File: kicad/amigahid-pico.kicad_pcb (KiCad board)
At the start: 2 copper layers, 80 x 76.2 mm, 60 parts, among them J1 Amiga keyboard connector, J2 Conn_02x05_Top_Bottom, J3 Conn_02x05_Top_Bottom, J4 Conn_01x06, J5 Conn_01x04, Q1 BSS138, Q10 BSS138, Q11 BSS138, Q12 BSS138, Q13 BSS138, Q14 BSS138, Q15 BSS138, Q16 BSS138, Q17 BSS138, Q2 BSS138, Q3 BSS138, Q4 BSS138, Q5 BSS138, Q6 BSS138, Q7 BSS138, Q8 BSS138, Q9 BSS138, U1 Pico

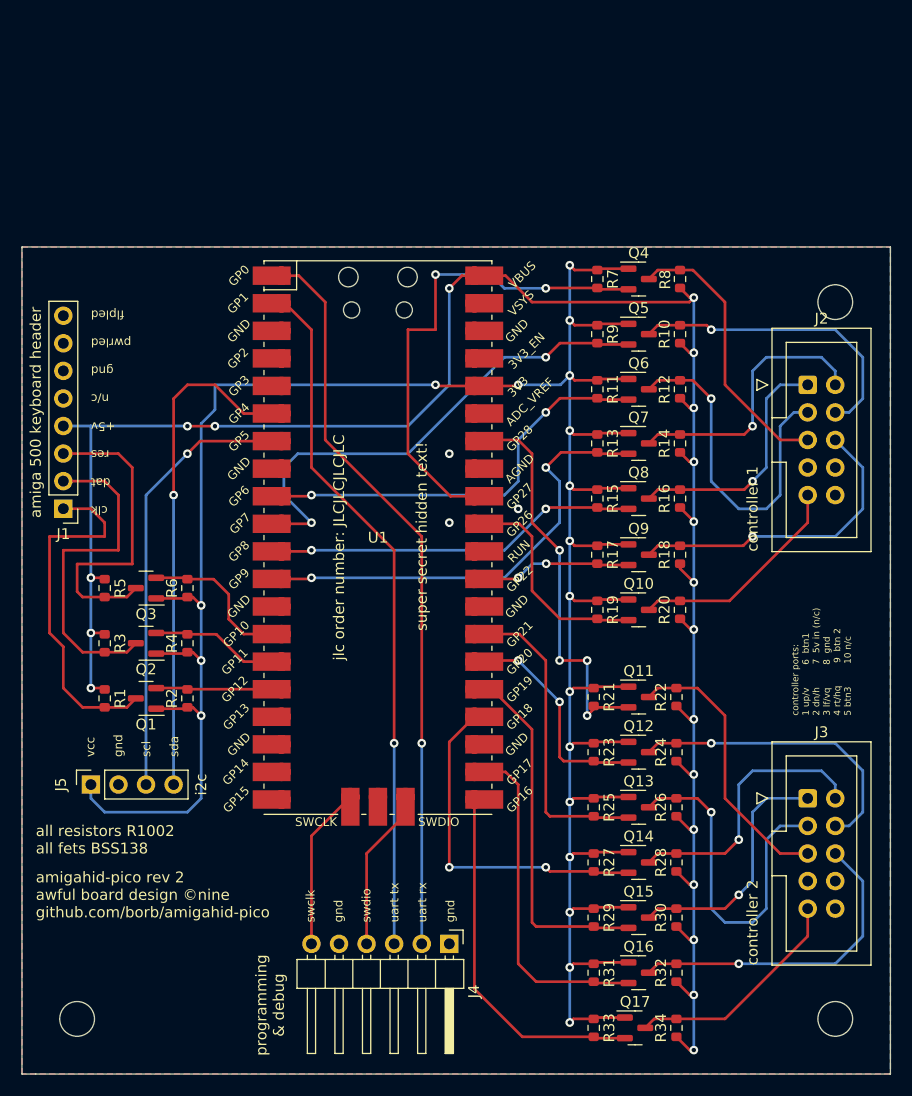
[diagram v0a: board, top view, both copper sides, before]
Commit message: pcb rev 4
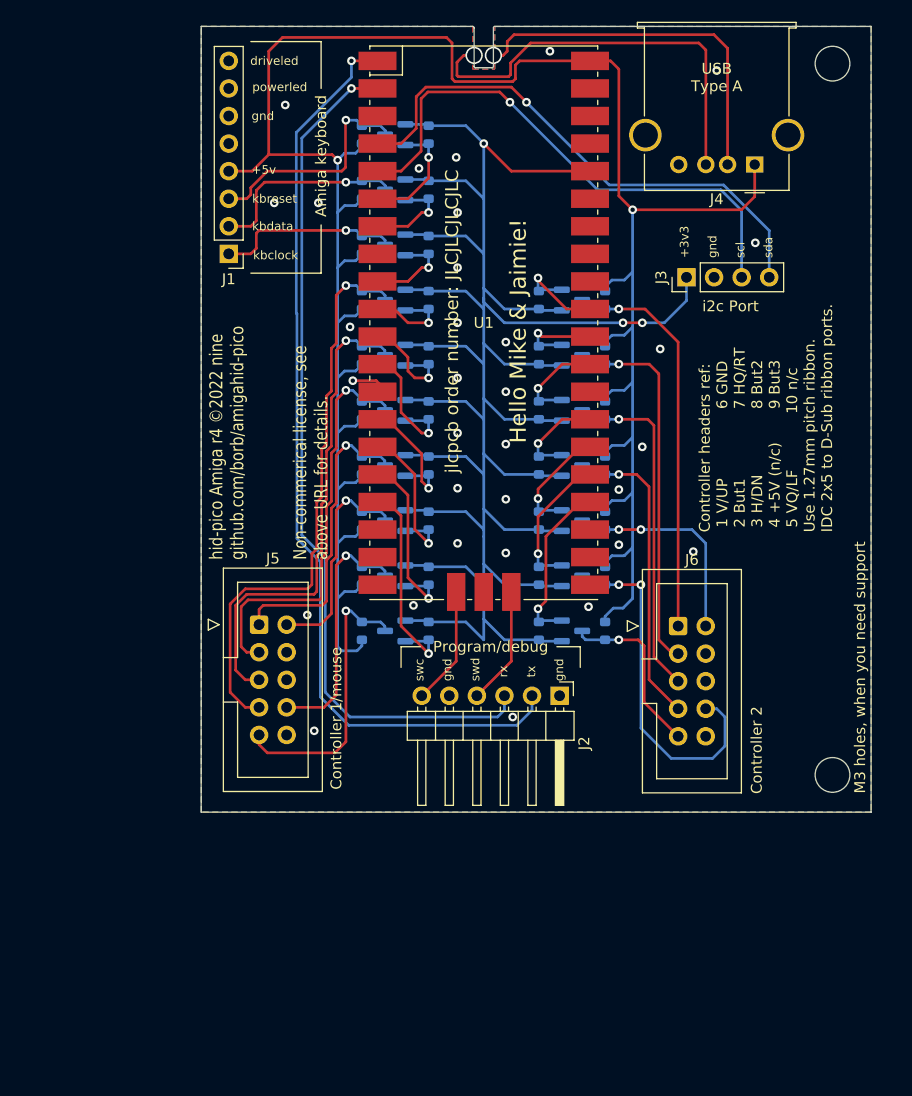
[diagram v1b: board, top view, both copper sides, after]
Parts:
- removed R15: R1002, Resistor_SMD:R_0603_1608Metric
- removed the REF** at (109.2, 135.9)
- removed the REF** at (179.1, 69.8)
- removed the REF** at (179.1, 135.9)
- added J6: Controller 2, Connector_IDC:IDC-Header_2x05_P2.54mm_Vertical, F.Cu at (164.6, 99.7)
- added REF**: MountingHole_3.2mm_M3, MountingHole:MountingHole_3.2mm_M3, F.Cu at (178.8, 47.9)
- added REF**: MountingHole_3.2mm_M3, MountingHole:MountingHole_3.2mm_M3, F.Cu at (178.8, 113.4)
- added locked: R1002, Resistor_SMD:R_0603_1608Metric, B.Cu at (135.5, 90.0)
- J1: value Amiga keyboard connector -> Amiga Keyboard
- J2: value Conn_02x05_Top_Bottom -> Debug/programming; footprint Connector_IDC:IDC-Header_2x05_P2.54mm_Vertical -> Connector_PinHeader_2.54mm:PinHeader_1x06_P2.54mm_Horizontal
- J3: value Conn_02x05_Top_Bottom -> i2c header; footprint Connector_IDC:IDC-Header_2x05_P2.54mm_Vertical -> Connector_PinHeader_2.54mm:PinHeader_1x04_P2.54mm_Vertical
- J4: value Conn_01x06 -> USB_A; footprint Connector_PinHeader_2.54mm:PinHeader_1x06_P2.54mm_Horizontal -> Connector_USB:USB_A_Molex_67643_Horizontal
- J5: value Conn_01x04 -> Controller 1; footprint Connector_PinSocket_2.54mm:PinSocket_1x04_P2.54mm_Vertical -> Connector_IDC:IDC-Header_2x05_P2.54mm_Vertical
- Q1, Q10, Q11, Q12, Q13, Q14, Q15, Q16, Q17, Q2, Q3, Q4, Q5, Q6, Q7, Q8, Q9, R1, R10, R11, R12, R13, R14, R16, R17, R18, R19, R2, R20, R21, R22, R23, R24, R25, R26, R27, R28, R29, R3, R30, R31, R32, R33, R34, R4, R5, R6, R7, R8, R9: moved to B.Cu
- moved J4 77.1 mm to (171.6, 57.2), turned to 180 degrees
- moved J3 49.3 mm to (165.4, 67.6), turned to 90 degrees
- moved R1 48.0 mm to (135.5, 64.6)
- moved R5 48.0 mm to (135.5, 54.4)
- moved R3 48.0 mm to (135.5, 59.5)
- moved Q1 47.7 mm to (138.5, 64.6)
- moved Q2 47.7 mm to (138.5, 59.5)
- moved Q3 47.7 mm to (138.5, 54.4)
- moved R2 47.3 mm to (141.6, 64.6)
- moved R6 47.3 mm to (141.6, 54.4)
- moved R4 47.3 mm to (141.6, 59.5)
- moved R22 38.7 mm to (151.8, 69.7), turned to -90 degrees
- moved R24 38.7 mm to (151.8, 74.7), turned to -90 degrees
- moved R26 38.7 mm to (151.8, 79.8), turned to -90 degrees
- moved R30 38.7 mm to (151.8, 90.0), turned to -90 degrees
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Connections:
- J1 pad 1: Net-(J1-Pad1) -> /kbclock
- J1 pad 2: Net-(J1-Pad2) -> /kbdata
- J1 pad 3: Net-(J1-Pad3) -> /kbreset
- J1 pad 4: /+5V -> +5V
- J1 pad 7: unconnected-(J1-Pad7) -> /kbpowerled
- J1 pad 8: unconnected-(J1-Pad8) -> /kbdriveled
- J2 pad 1: Net-(J2-Pad1) -> GND
- J2 pad 2: Net-(J2-Pad2) -> /uart tx
- J2 pad 3: Net-(J2-Pad3) -> /uart rx
- J2 pad 4: Net-(J2-Pad4) -> /swdio
- J2 pad 5: Net-(J2-Pad5) -> GND
- J2 pad 6: Net-(J2-Pad6) -> /swclk
- J3 pad 1: Net-(J3-Pad1) -> +3V3
- J3 pad 2: Net-(J3-Pad2) -> GND
- J3 pad 3: Net-(J3-Pad3) -> /i2c scl
- J3 pad 4: Net-(J3-Pad4) -> /i2c sda
- J4 pad 1: GND -> +5V
- J4 pad 2: Net-(J4-Pad2) -> /usb d-
- J4 pad 3: Net-(J4-Pad3) -> /usb d+
- J4 pad 4: Net-(J4-Pad4) -> GND
- J5 pad 1: +3V3 -> /cont1 v
- J5 pad 2: GND -> /cont1 b1
- J5 pad 3: Net-(J5-Pad3) -> /cont1 h
- J5 pad 4: Net-(J5-Pad4) -> unconnected-(J5-Pad4)
- Q1 pad 2: Net-(Q1-Pad2) -> /lkbclock
- Q1 pad 3: Net-(J1-Pad1) -> /kbclock
- Q10 pad 2: Net-(Q10-Pad2) -> /lcont1 b3
- Q10 pad 3: Net-(J2-Pad9) -> /cont1 b3
- Q11 pad 2: Net-(Q11-Pad2) -> /lcont2 v
- Q11 pad 3: Net-(J3-Pad5) -> /cont2 v
- Q12 pad 2: Net-(Q12-Pad2) -> /lcont2 h
- Q12 pad 3: Net-(J3-Pad4) -> /cont2 h
- Q13 pad 2: Net-(Q13-Pad2) -> /lcont2 vq
- Q13 pad 3: Net-(J3-Pad3) -> /cont2 vq
- Q14 pad 2: Net-(Q14-Pad2) -> /lcont2 hq
- Q14 pad 3: Net-(J3-Pad2) -> /cont2 hq
- Q15 pad 2: Net-(Q15-Pad2) -> /lcont2 b1
- Q15 pad 3: Net-(J3-Pad1) -> /cont2 b1
- Q16 pad 2: Net-(Q16-Pad2) -> /lcont2 b2
- Q16 pad 3: Net-(J3-Pad6) -> /cont2 b2
- Q17 pad 2: Net-(Q17-Pad2) -> /lcont2 b3
- Q17 pad 3: Net-(J3-Pad9) -> /cont2 b3
- Q2 pad 2: Net-(Q2-Pad2) -> /lkbdata
- Q2 pad 3: Net-(J1-Pad2) -> /kbdata
- Q3 pad 2: Net-(Q3-Pad2) -> /lkbreset
- Q3 pad 3: Net-(J1-Pad3) -> /kbreset
- Q4 pad 2: Net-(Q4-Pad2) -> /lcont1 hq
- Q4 pad 3: Net-(J2-Pad5) -> /cont1 hq
- Q5 pad 2: Net-(Q5-Pad2) -> /lcont1 vq
- Q5 pad 3: Net-(J2-Pad4) -> /cont1 vq
- Q6 pad 2: Net-(Q6-Pad2) -> /lcont1 h
- Q6 pad 3: Net-(J2-Pad3) -> /cont1 h
- Q7 pad 2: Net-(Q7-Pad2) -> /lcont1 v
- Q7 pad 3: Net-(J2-Pad2) -> /cont1 v
- Q8 pad 2: Net-(Q8-Pad2) -> /lcont1 b1
- Q8 pad 3: Net-(J2-Pad1) -> /cont1 b1
- Q9 pad 2: Net-(Q9-Pad2) -> /lcont1 b2
- Q9 pad 3: Net-(J2-Pad6) -> /cont1 b2
- R1 pad 1: /+5V -> /kbclock
- R1 pad 2: Net-(J1-Pad1) -> +5V
- R10 pad 1: /+5V -> /lcont1 vq
- R10 pad 2: Net-(J2-Pad4) -> +3V3
- R11 pad 1: +3V3 -> /cont1 h
- R11 pad 2: Net-(Q6-Pad2) -> +5V
- R12 pad 1: /+5V -> /lcont1 h
- R12 pad 2: Net-(J2-Pad3) -> +3V3
- R13 pad 1: +3V3 -> /cont1 v
- R13 pad 2: Net-(Q7-Pad2) -> +5V
- R14 pad 1: /+5V -> /lcont1 v
- R14 pad 2: Net-(J2-Pad2) -> +3V3
- R16 pad 1: /+5V -> /lcont1 b1
- R16 pad 2: Net-(J2-Pad1) -> +3V3
- R17 pad 1: +3V3 -> /cont1 b2
- R17 pad 2: Net-(Q9-Pad2) -> +5V
- R18 pad 1: /+5V -> /lcont1 b2
- R18 pad 2: Net-(J2-Pad6) -> +3V3
- R19 pad 1: +3V3 -> /cont1 b3
- R19 pad 2: Net-(Q10-Pad2) -> +5V
- R2 pad 1: +3V3 -> /lkbclock
- R2 pad 2: Net-(Q1-Pad2) -> +3V3
- R20 pad 1: /+5V -> /lcont1 b3
- R20 pad 2: Net-(J2-Pad9) -> +3V3
- R21 pad 1: +3V3 -> /cont2 v
- R21 pad 2: Net-(Q11-Pad2) -> +5V
- R22 pad 1: /+5V -> /lcont2 v
- R22 pad 2: Net-(J3-Pad5) -> +3V3
- R23 pad 1: +3V3 -> /cont2 h
- R23 pad 2: Net-(Q12-Pad2) -> +5V
- R24 pad 1: /+5V -> /lcont2 h
- R24 pad 2: Net-(J3-Pad4) -> +3V3
- R25 pad 1: +3V3 -> /cont2 vq
- R25 pad 2: Net-(Q13-Pad2) -> +5V
- R26 pad 1: /+5V -> /lcont2 vq
- R26 pad 2: Net-(J3-Pad3) -> +3V3
- R27 pad 1: +3V3 -> /cont2 hq
- R27 pad 2: Net-(Q14-Pad2) -> +5V
- R28 pad 1: /+5V -> /lcont2 hq
- R28 pad 2: Net-(J3-Pad2) -> +3V3
- R29 pad 1: +3V3 -> /cont2 b1
- R29 pad 2: Net-(Q15-Pad2) -> +5V
- R3 pad 1: /+5V -> /kbdata
- R3 pad 2: Net-(J1-Pad2) -> +5V
- R30 pad 1: /+5V -> /lcont2 b1
- R30 pad 2: Net-(J3-Pad1) -> +3V3
- R31 pad 1: +3V3 -> /cont2 b2
- R31 pad 2: Net-(Q16-Pad2) -> +5V
- R32 pad 1: /+5V -> /lcont2 b2
- R32 pad 2: Net-(J3-Pad6) -> +3V3
- R33 pad 1: +3V3 -> /cont2 b3
- R33 pad 2: Net-(Q17-Pad2) -> +5V
- R34 pad 1: /+5V -> /lcont2 b3
- R34 pad 2: Net-(J3-Pad9) -> +3V3
- R4 pad 1: +3V3 -> /lkbdata
- R4 pad 2: Net-(Q2-Pad2) -> +3V3
- R5 pad 1: /+5V -> /kbreset
- R5 pad 2: Net-(J1-Pad3) -> +5V
- R6 pad 1: +3V3 -> /lkbreset
- R6 pad 2: Net-(Q3-Pad2) -> +3V3
- R7 pad 1: +3V3 -> /cont1 hq
- R7 pad 2: Net-(Q4-Pad2) -> +5V
- R8 pad 1: /+5V -> /lcont1 hq
- R8 pad 2: Net-(J2-Pad5) -> +3V3
- R9 pad 1: +3V3 -> /cont1 vq
- R9 pad 2: Net-(Q5-Pad2) -> +5V
- U1 pad 1: Net-(J4-Pad2) -> /uart tx
- U1 pad 10: Net-(Q5-Pad2) -> /lcont1 hq
- U1 pad 11: Net-(Q8-Pad2) -> /lcont1 vq
- U1 pad 12: Net-(Q7-Pad2) -> /lcont1 h
- U1 pad 14: Net-(Q3-Pad2) -> /lcont1 v
- U1 pad 15: Net-(Q2-Pad2) -> /lcont1 b1
- U1 pad 16: Net-(Q1-Pad2) -> /lcont1 b2
- U1 pad 17: unconnected-(U1-Pad17) -> /lcont1 b3
- U1 pad 2: Net-(J4-Pad3) -> /uart rx
- U1 pad 21: Net-(Q17-Pad2) -> unconnected-(U1-Pad21)
- U1 pad 22: Net-(Q16-Pad2) -> unconnected-(U1-Pad22)
- U1 pad 24: Net-(Q14-Pad2) -> /lcont2 b3
- U1 pad 25: Net-(Q15-Pad2) -> /lcont2 b2
- U1 pad 26: Net-(Q12-Pad2) -> /lcont2 b1
- U1 pad 27: Net-(Q13-Pad2) -> /lcont2 hq
- U1 pad 29: Net-(Q9-Pad2) -> /lcont2 vq
- U1 pad 30: unconnected-(U1-Pad30) -> /lcont2 h
- U1 pad 31: Net-(Q10-Pad2) -> /lcont2 v
- U1 pad 32: Net-(Q4-Pad2) -> unconnected-(U1-Pad32)
- U1 pad 34: Net-(Q11-Pad2) -> unconnected-(U1-Pad34)
- U1 pad 4: unconnected-(U1-Pad4) -> /i2c sda
- U1 pad 40: /+5V -> +5V
- U1 pad 41: Net-(J4-Pad6) -> /swclk
- U1 pad 43: Net-(J4-Pad4) -> /swdio
- U1 pad 5: unconnected-(U1-Pad5) -> /i2c scl
- U1 pad 6: Net-(J5-Pad4) -> /lkbreset
- U1 pad 7: Net-(J5-Pad3) -> /lkbdata
- U1 pad 9: Net-(Q6-Pad2) -> /lkbclock
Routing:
- net +5V: track 0.00 -> 220.3 mm, vias 0 -> 2
- net /+5V: track 194.7 -> 0.00 mm, vias 20 -> 0
- net /uart tx: track 0.00 -> 87.4 mm, vias 0 -> 1
- net /uart rx: track 0.00 -> 80.8 mm, vias 0 -> 1
- net Net-(J4-Pad2): track 67.9 -> 0.00 mm, vias 1 -> 0
- net Net-(J4-Pad3): track 63.5 -> 0.00 mm, vias 1 -> 0
- net /cont1 hq: track 0.00 -> 52.9 mm, vias 0 -> 1
- net /i2c scl: track 0.00 -> 49.2 mm, vias 0 -> 1
- net /i2c sda: track 0.00 -> 48.8 mm, vias 0 -> 1
- net Net-(J5-Pad4): track 47.1 -> 0.00 mm, vias 1 -> 0
- net Net-(Q5-Pad2): track 45.5 -> 0.00 mm, vias 2 -> 0
- net Net-(Q4-Pad2): track 45.2 -> 0.00 mm, vias 2 -> 0
- net /cont1 vq: track 0.00 -> 45.1 mm, vias 0 -> 1
- net Net-(Q7-Pad2): track 41.6 -> 0.00 mm, vias 2 -> 0
- net Net-(J5-Pad3): track 41.2 -> 0.00 mm, vias 1 -> 0
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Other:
- board size 80 x 76.2 mm -> 61.7 x 72.4 mm
- board text added: "+3v3 gnd scl sda"
- board text added: "+5v"
- board text added: "6 GND 7 HQ/RT 8 But2 9 But3 10 n/c"
- board text added: "All FETs (Q*) part BSS138 All resistors (R*) part R1002"
- board text added: "Amiga keyboard"
- board text added: "Controller 1/mouse"
- board text added: "Controller 2"
- board text added: "Controller headers ref: 1 V/UP 2 But1 3 H/DN 4 +5V (n/c) 5 VQ/LF Use 1.27mm pitch ribbon. IDC 2x5 to D-Sub ribbon ports."
- board text added: "Hello Mike & Jaimie!"
- board text added: "M3 holes, when you need support"
- board text added: "Program/debug"
- board text added: "Solder VERY carefully to --> enable USB Type A port. Pico test pads are very close to shield (ground) solder points."
- board text added: "USB Type A"
- board text added: "driveled"
- board text added: "gnd"
- board text added: "hid-pico Amiga r4 ©️2022 nine github.com/borb/amigahid-pico Non-commerical license, see above URL for details."
- board text added: "i2c Port"
- board text added: "jlcpcb order number: JLCJLCJLCJLC"
- board text added: "kbclock"
- board text added: "kbdata"
- board text added: "kbreset"
- board text added: "powerled"
- board text added: "swc gnd swd rx tx gnd"
- board text removed: "all resistors R1002 all fets BSS138"
- board text removed: "amiga 500 keyboard header"
- board text removed: "amigahid-pico rev 2 awful board design ©nine github.com/borb/amigahid-pico"
- board text removed: "clk dat res +5v n/c gnd pwrled flpled"
- board text removed: "controller 1"
- board text removed: "controller 2"
- board text removed: "controller ports: 1 up/v 6 btn1 2 dn/h 7 5v in (n/c) 3 lf/vq 8 gnd 4 rt/hq 9 btn 2 5 btn3 10 n/c"
- board text removed: "i2c"
- board text removed: "jlc order number: JLCJLCJLCJLC"
- board text removed: "programming & debug"
- board text removed: "super secret hidden text!"
- board text removed: "swclk gnd swdio uart tx uart rx gnd"
- board text removed: "vcc gnd scl sda"
